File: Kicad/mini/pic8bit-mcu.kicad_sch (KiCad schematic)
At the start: 30 parts, among them K201 *Power & UART, K202 MCU 1, K203 MCU 1, K204 ICSP, K205 MCU 2, K206 MCU 2, U201 TLV1117-33, U202 PIC16F/PIC18F

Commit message: Up
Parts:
- removed C204: 10µ, tronixio:KEMET-C322, symbol tronixio:KEMET-C322-0508-10U-25V-10P
- added C204: 10µ, tronixio:CAPACITOR-SMD-1206, symbol tronixio:CAPACITOR-1206-10U-25V-5P-X7R
- K201: footprint tronixio:FCI-USB-TYPE-B-MICRO-THT -> tronixio:USB-TYPE-B-MICRO-TH
- U202: footprint tronixio:DIP-28-W762 -> tronixio:DIP-28-W762-SOCKET
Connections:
- net GND: now also K201.SH (SHIELD), C204.2; no longer K201.6 (SHIELD)
- net at JP203.2: now also C204.1
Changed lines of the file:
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@@
+    )
+  )
+  (symbol (lib_id "tronixio:CAPACITOR-1206-10U-25V-5P-X7R") (at 119.38 104.14 0) (unit 1)
+    (in_bom yes) (on_board yes) (dnp no)
+    (property "Reference" "C204" (at 118.745 106.68 0)
+      (effects (font (size 1.15 1.15)) (justify right))
+    )
+    (property "Value" "10µ" (at 118.745 109.22 0)
+      (effects (font (size 1.15 1.15)) (justify right))
+    )
+    (property "Footprint" "tronixio:CAPACITOR-SMD-1206" (at 119.38 114.3 0) (do_not_autoplace)
+      (effects (font (size 1 1)) hide)
+    )
+    (property "Datasheet" "" (at 119.38 119.38 0)
+      (effects (font (size 1 1)) hide)
+    )
+    (property "Tolerance" "5%" (at 120.38 109.22 0) (do_not_autoplace)
+      (effects (font (size 1.15 1.15)) (justify left) hide)
+    )
+    (property "Mouser" "791-1206X106J250CT" (at 119.38 116.84 0) (do_not_autoplace)
+      (effects (font (size 1 1)) hide)
+    )
+    (property "Voltage" "25V" (at 124.38 109.22 0) (do_not_autoplace)
+      (effects (font (size 1.15 1.15)) (justify left) hide)
+    )
+    (pin "1")
+    (pin "2")
+    (instances
+      (project "pic8bit"
+        (path "/d431d485-8cd8-4e00-afcd-f39218d614ca/64edc06d-d6ae-4dac-9759-3f1fbed6457d"
+          (reference "C204") (unit 1)
+        )
+      )
     )
   )
@@
       (effects (font (size 1.15 1.15)))
     )
-    (property "Footprint" "tronixio:FCI-USB-TYPE-B-MICRO-THT" (at 38.1 193.04 0) (do_not_autoplace)
+    (property "Footprint" "tronixio:USB-TYPE-B-MICRO-TH" (at 38.1 193.04 0) (do_not_autoplace)
       (effects (font (size 1 1)) hide)
     )
@@
     (pin "4")
     (pin "5")
-    (pin "6")
+    (pin "SH")
     (instances
       (project "pic8bit"
@@
       (effects (font (size 1.15 1.15)) (justify right))
     )
-    (property "Footprint" "tronixio:DIP-28-W762" (at 144.78 96.52 0) (do_not_autoplace)
+    (property "Footprint" "tronixio:DIP-28-W762-SOCKET" (at 144.78 96.52 0) (do_not_autoplace)
       (effects (font (size 1 1)) hide)
     )
@@
         )
       )
-    )
-  )
-  (symbol (lib_id "tronixio:KEMET-C322-0508-10U-25V-10P") (at 119.38 104.14 0) (unit 1)
-    (in_bom yes) (on_board yes) (dnp no)
-    (property "Reference" "C204" (at 118.745 106.68 0)
-      (effects (font (size 1.15 1.15)) (justify right))
-    )
-    (property "Value" "10µ" (at 118.745 109.22 0)
-      (effects (font (size 1.15 1.15)) (justify right))
-    )
-    (property "Footprint" "tronixio:KEMET-C322" (at 119.38 116.84 0) (do_not_autoplace)
-      (effects (font (size 1 1)) hide)
-    )
-    (property "Datasheet" "https://content.kemet.com/datasheets/KEM_C1054_HIVOLT_GOLDMAX_300_C0G.pdf" (at 119.38 114.3 0) (do_not_autoplace)
-      (effects (font (size 1 1)) hide)
-    )
-    (property "Tolerance" "10%" (at 124.46 109.22 0) (do_not_autoplace)
-      (effects (font (size 1.15 1.15)) (justify left) hide)
-    )
-    (property "Mouser" "80-C322C106K3R" (at 119.38 119.38 0) (do_not_autoplace)
-      (effects (font (size 1 1)) hide)
-    )
-    (property "Voltage" "25V" (at 120.65 109.22 0) (do_not_autoplace)
-      (effects (font (size 1.15 1.15)) (justify left) hide)
-    )
-    (pin "1")
-    (pin "2")
-    (instances
-      (project "pic8bit"
-        (path "/d431d485-8cd8-4e00-afcd-f39218d614ca/64edc06d-d6ae-4dac-9759-3f1fbed6457d"
-          (reference "C204") (unit 1)
-        )
-      )

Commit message: Up
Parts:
- K201: symbol tronixio:FCI-USB-TYPE-B-MICRO-THT -> tronixio:FCI-USB-TYPE-B-MICRO-TH
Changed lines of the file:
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@@
     )
   )
-  (symbol (lib_id "tronixio:FCI-USB-TYPE-B-MICRO-THT") (at 38.1 175.26 0) (unit 1)
+  (symbol (lib_id "tronixio:FCI-USB-TYPE-B-MICRO-TH") (at 38.1 175.26 0) (unit 1)
     (in_bom yes) (on_board yes) (dnp no)
     (property "Reference" "K201" (at 38.1 162.56 0)

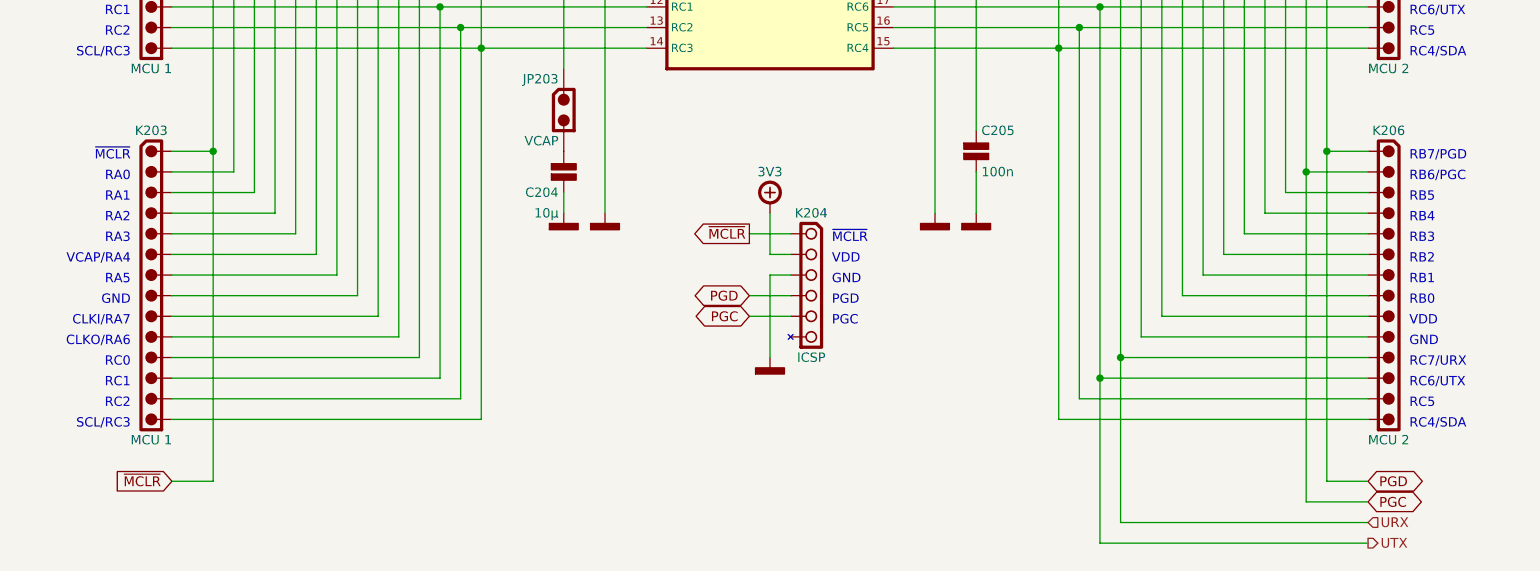
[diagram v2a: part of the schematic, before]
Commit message: Up
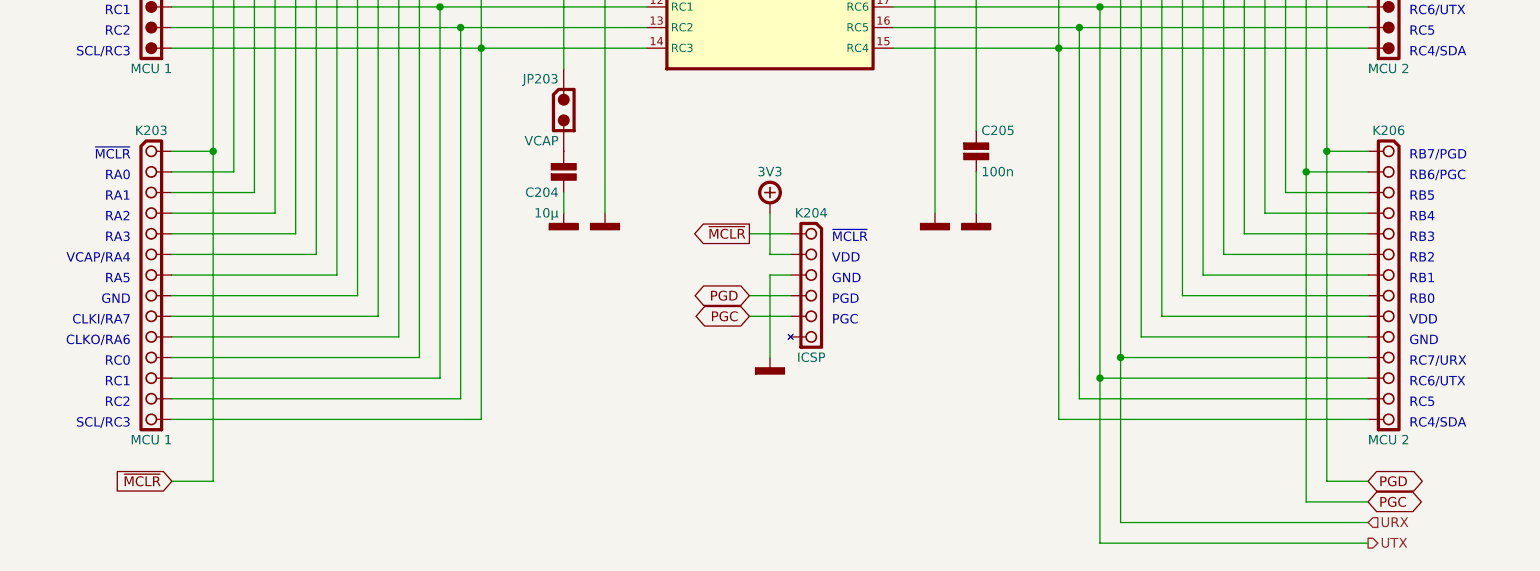
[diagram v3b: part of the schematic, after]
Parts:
- K204: symbol tronixio:MICROCHIP-ICSP-F-1X06 -> tronixio:MICROCHIP-ICSP-F-RIGHT-ANGLE-TH
- U202: footprint tronixio:DIP-28-W762-SOCKET -> tronixio:DIP-28-W762
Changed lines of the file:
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@@
       (effects (font (size 1.15 1.15)) (justify right))
     )
-    (property "Footprint" "tronixio:DIP-28-W762-SOCKET" (at 144.78 96.52 0) (do_not_autoplace)
+    (property "Footprint" "tronixio:DIP-28-W762" (at 144.78 96.52 0) (do_not_autoplace)
       (effects (font (size 1 1)) hide)
     )
@@
     )
   )
-  (symbol (lib_id "tronixio:MICROCHIP-ICSP-F-1X06") (at 149.86 111.76 0) (unit 1)
+  (symbol (lib_id "tronixio:MICROCHIP-ICSP-F-RIGHT-ANGLE-TH") (at 149.86 111.76 0) (unit 1)
     (in_bom yes) (on_board yes) (dnp no)
     (property "Reference" "K204" (at 149.86 109.22 0)

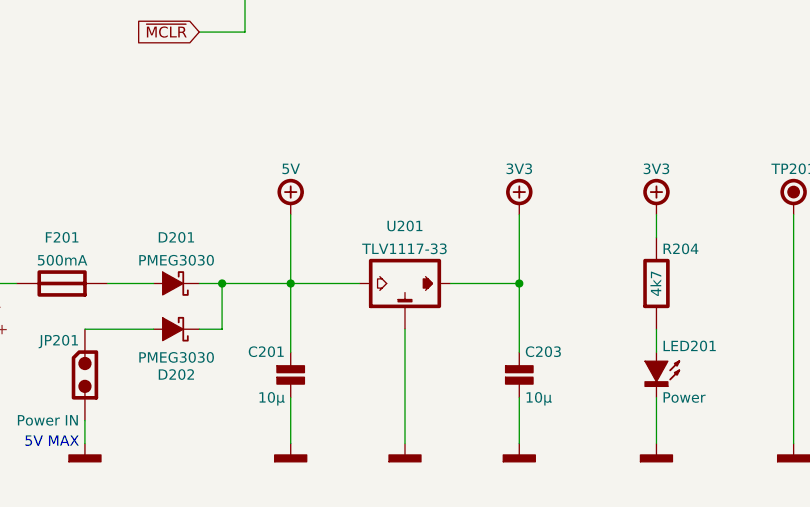
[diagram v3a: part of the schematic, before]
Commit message: Update
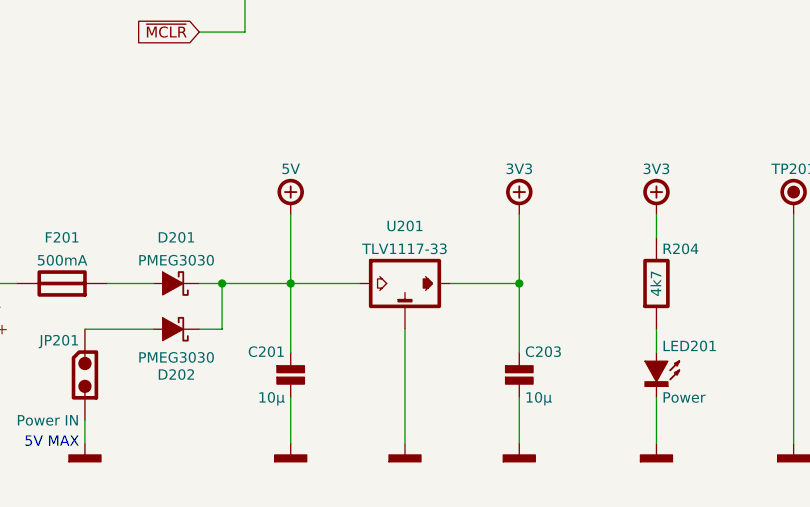
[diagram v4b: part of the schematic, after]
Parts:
- C201, C203, C204: Mouser 791-1206X106J250CT -> 80-C1206C106J3R
- D201, D202: symbol tronixio:NEXPERIA-PMEG3030 -> tronixio:NEXPERIA-PMEG3030-SOD
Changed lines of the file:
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@@
       (effects (font (size 1.15 1.15)) (justify left) hide)
     )
-    (property "Mouser" "791-1206X106J250CT" (at 119.38 116.84 0) (do_not_autoplace)
+    (property "Mouser" "80-C1206C106J3R" (at 119.38 116.84 0) (do_not_autoplace)
       (effects (font (size 1 1)) hide)
     )
@@
     )
   )
-  (symbol (lib_id "tronixio:NEXPERIA-PMEG3030") (at 68.58 175.26 180) (unit 1)
+  (symbol (lib_id "tronixio:NEXPERIA-PMEG3030-SOD") (at 68.58 175.26 180) (unit 1)
     (in_bom yes) (on_board yes) (dnp no)
     (property "Reference" "D202" (at 68.58 180.34 0)
@@
       (effects (font (size 1.15 1.15)) (justify left) hide)
     )
-    (property "Mouser" "791-1206X106J250CT" (at 81.28 193.04 0) (do_not_autoplace)
+    (property "Mouser" "80-C1206C106J3R" (at 81.28 193.04 0) (do_not_autoplace)
       (effects (font (size 1 1)) hide)
     )
@@
       (effects (font (size 1.15 1.15)) (justify left) hide)
     )
-    (property "Mouser" "791-1206X106J250CT" (at 106.68 193.04 0) (do_not_autoplace)
+    (property "Mouser" "80-C1206C106J3R" (at 106.68 193.04 0) (do_not_autoplace)
       (effects (font (size 1 1)) hide)
     )
@@
     )
   )
-  (symbol (lib_id "tronixio:NEXPERIA-PMEG3030") (at 68.58 170.18 180) (unit 1)
+  (symbol (lib_id "tronixio:NEXPERIA-PMEG3030-SOD") (at 68.58 170.18 180) (unit 1)
     (in_bom yes) (on_board yes) (dnp no)
     (property "Reference" "D201" (at 68.58 165.1 0)
